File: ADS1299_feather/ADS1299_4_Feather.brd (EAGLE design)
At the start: 90 x 40 mm, 40 parts, among them U1 ADS1299-4PAG

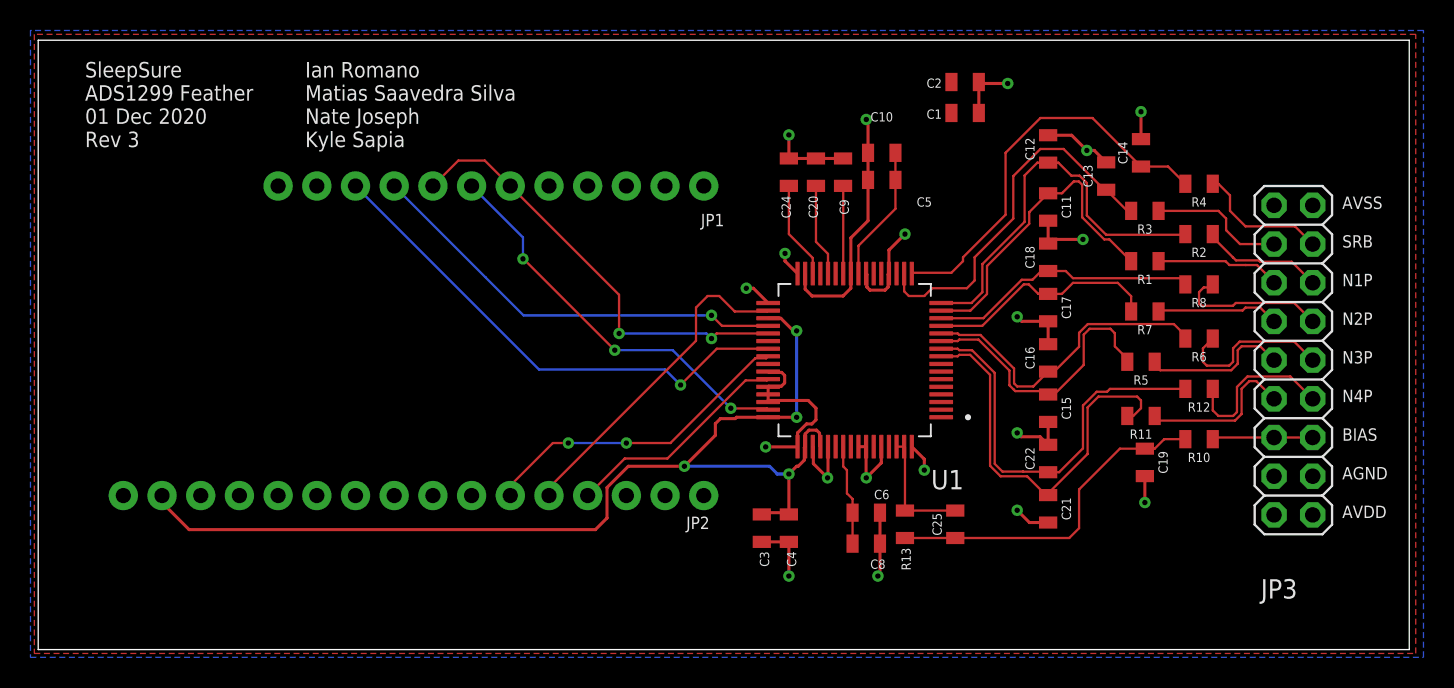
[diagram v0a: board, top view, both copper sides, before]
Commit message: Uploading final standalone and feather files
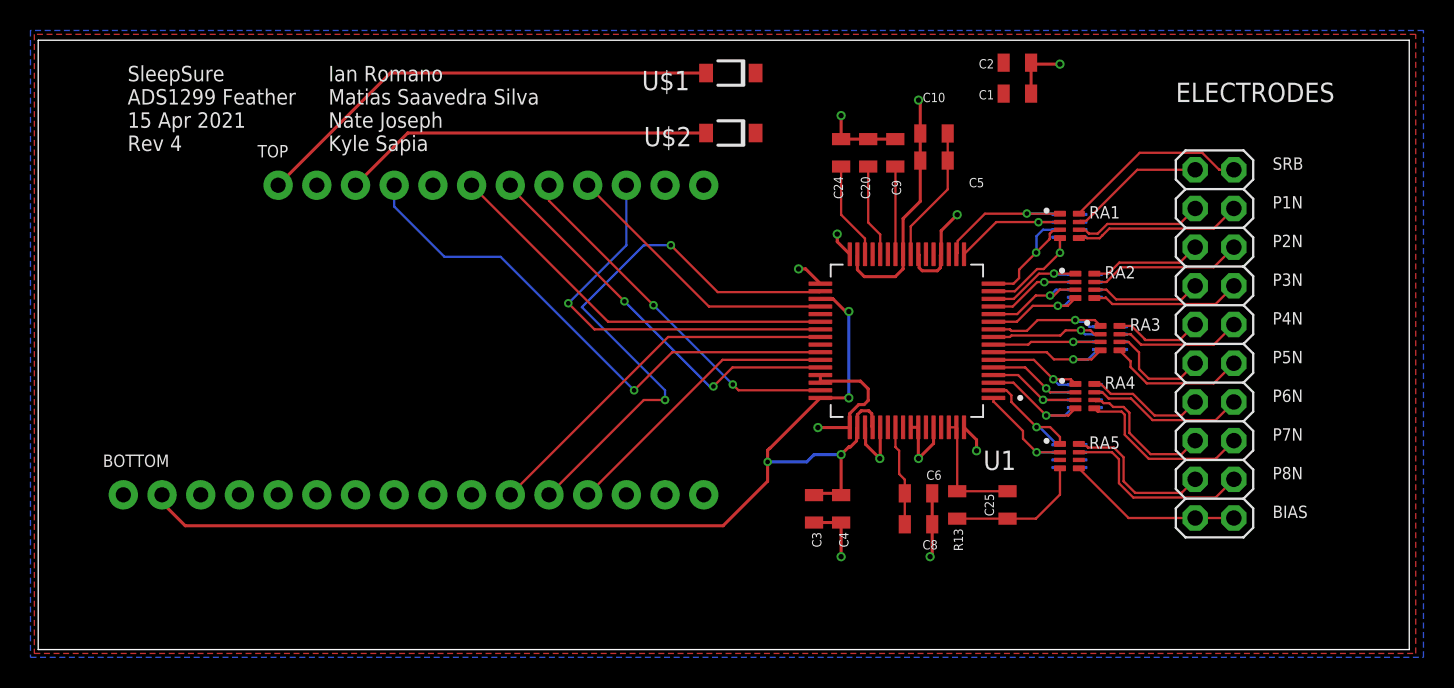
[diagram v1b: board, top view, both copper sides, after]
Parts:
- removed C11, C12, C13, C14, C15, C16, C17, C18, C19, C21, C22: 1nF, SparkFun-Capacitors:0805
- removed JP1: 1x12, Proto FeatherWing:MICROBUILDER_1X12_ROUND_76MIL
- removed JP2: 1x16, Proto FeatherWing:MICROBUILDER_1X16_ROUND_76MIL
- removed JP3: 2x9, adafruit:2X09-BIG
- removed R1, R10, R11, R12, R2, R3, R4, R5, R6, R7, R8: 2.2k, SparkFun-Resistors:0805
- added BOTTOM: (no value), ADS_Feather:MICROBUILDER_1X16_ROUND_76MIL
- added CA1, CA2, CA3, CA4, CA5: 1nF, ADS_Feather:SLEEPSURELIB_CAPCAXE50P210X130X94-8N
- added ELECTRODES: (no value), ADS_Feather:SLEEPSURELIB_2X10-BIG
- added RA1, RA2, RA3, RA4, RA5: 2.2k, ADS_Feather:SLEEPSURELIB_RESCAXS50P200X100X45-8N
- added TOP: (no value), ADS_Feather:MICROBUILDER_1X12_ROUND_76MIL
- added U$1, U$2: MRB120, ADS_Feather:SOD123FL
- moved C10 3.66 mm to (58.8, 33.9)
- moved C5 3.66 mm to (58.8, 32.1)
- moved C25 3.66 mm to (63.6, 9.49)
- moved C3 3.66 mm to (50.9, 9.24)
- moved R13 3.66 mm to (60.3, 9.49)
- moved U1 3.66 mm to (57.0, 20.3)
- moved C9 3.66 mm to (56.3, 32.6)
- moved C2 3.66 mm to (64.3, 38.5)
- moved C4 3.66 mm to (52.7, 9.24)
- moved C8 3.66 mm to (57.8, 8.22)
- moved C6 3.66 mm to (57.8, 10.3)
- moved C1 3.66 mm to (64.3, 36.5)
- moved C20 3.66 mm to (54.5, 32.6)
- moved C24 3.66 mm to (52.7, 32.6)
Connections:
- removed net CLK0: JP1.6, JP1.8, U1.37
- removed net EN: JP1.2
- removed net RESET: JP2.1
- new net 5_N: ELECTRODES.N5, RA3.5
- new net 5_P: ELECTRODES.P5, RA3.6
- new net 6_N: ELECTRODES.N6, RA4.7
- new net 6_P: ELECTRODES.P6, RA4.8
- new net 7_N: ELECTRODES.N7, RA4.5
- new net 7_P: ELECTRODES.P7, RA4.6
- new net 8_N: ELECTRODES.N8, RA5.7
- new net 8_P: ELECTRODES.P8, RA5.8
- new net ADS_START: TOP.27/A10, U1.38
- new net GPIO1: TOP.13/A12, U1.42
- new net GPIO2: TOP.33/A9, U1.44
- new net IN5_N: CA3.1, RA3.4, U1.7
- new net IN5_P: CA3.2, RA3.3, U1.8
- new net IN6_N: CA4.3, RA4.2, U1.5
- new net IN6_P: CA4.4, RA4.1, U1.6
- new net IN7_N: CA4.1, RA4.4, U1.3
- new net IN7_P: CA4.2, RA4.3, U1.4
- new net IN8_N: CA5.3, RA5.2, U1.1
- new net IN8_P: CA5.4, RA5.1, U1.2
- new net USB: TOP.USB, U$2.A
- net 1_N: now also ELECTRODES.N1, RA1.5; no longer JP3.14, R1.1
- net 1_P: now also ELECTRODES.P1, RA1.6; no longer JP3.13, R2.1
- net 2_N: now also ELECTRODES.N2, RA2.7; no longer JP3.12, R7.1
- net 2_P: now also ELECTRODES.P2, RA2.8; no longer JP3.11, R8.1
- net 3V3: now also BOTTOM.3V; no longer JP2.2
- net 3_N: now also ELECTRODES.N3, RA2.5; no longer JP3.10, R5.1
- net 3_P: now also ELECTRODES.P3, RA2.6; no longer JP3.9, R6.1
- net 4_N: now also ELECTRODES.N4, RA3.7; no longer JP3.8, R11.1
- net 4_P: now also ELECTRODES.P4, RA3.8; no longer JP3.7, R12.1
- net 5V: now also U$1.C, U$2.C; no longer JP1.3, JP3.1, JP3.2, U1.1, U1.2, U1.3, U1.4, U1.5, U1.6, U1.7, U1.8
- net ADS_RESET: now also TOP.32/A7; no longer JP1.9
- net BATT: now also TOP.BAT, U$1.A; no longer JP1.1
- net BIAS: now also ELECTRODES.BIAS1, ELECTRODES.BIAS2, RA5.5; no longer JP3.5, JP3.6, R10.1
- net BIAS_DRV: now also RA5.4; no longer C19.1, R10.2
- net CS1: now also TOP.14/A6; no longer JP1.10
- net DRDY: now also TOP.15/A8; no longer JP1.7
- net GND: now also BOTTOM.GND, CA1.5, CA1.6, CA1.7, CA1.8, CA2.5, CA2.6, CA2.7, CA2.8, CA3.5, CA3.6, CA3.7, CA3.8, CA4.5, CA4.6, CA4.7, CA4.8, CA5.5, CA5.6; no longer C11.2, C12.2, C13.2, C14.2, C15.2, C16.2, C17.2, C18.2, C19.2, C21.2, C22.2, JP2.4, JP3.17, JP3.18, JP3.3, JP3.4, U1.42, U1.44
- net IN1_N: now also CA1.1, RA1.4; no longer C11.1, R1.2
- net IN1_P: now also CA1.2, RA1.3; no longer C12.1, R2.2
- net IN2_N: now also CA2.3, RA2.2; no longer C17.1, R7.2
- net IN2_P: now also CA2.4, RA2.1; no longer C18.1, R8.2
- net IN3_N: now also CA2.1, RA2.4; no longer C15.1, R5.2
- net IN3_P: now also CA2.2, RA2.3; no longer C16.1, R6.2
- net IN4_N: now also CA3.3, RA3.2; no longer C21.1, R11.2
- net IN4_P: now also CA3.4, RA3.1; no longer C22.1, R12.2
- net MISO: now also BOTTOM.MISO/19; no longer JP2.13
- net MOSI: now also BOTTOM.MOSI/18; no longer JP2.12
- net SCLK: now also BOTTOM.SCK/5; no longer JP2.11
- net SRB1: now also ELECTRODES.SRB1, RA1.7; no longer JP3.15, R4.1
- net SRB2: now also ELECTRODES.SRB2, RA1.8; no longer JP3.16, R3.1
- net _SRB1: now also CA1.3, RA1.2; no longer C14.1, R4.2
- net _SRB2: now also CA1.4, RA1.1; no longer C13.1, R3.2
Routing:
- net GPIO1: track 0.00 -> 35.4 mm, vias 0 -> 1
- net BATT: track 0.00 -> 31.1 mm
- net CLK0: track 29.2 -> 0.00 mm, vias 2 -> 0
- net ADS_START: track 0.00 -> 26.6 mm
- net GPIO2: track 0.00 -> 26.4 mm, vias 0 -> 2
- net GND: track 89.0 -> 63.9 mm, vias 19 -> 12
- net USB: track 0.00 -> 24.4 mm
- net IN4_N: track 26.7 -> 8.54 mm, vias 0 -> 1
- net _SRB1: track 26.5 -> 8.42 mm, vias 0 -> 1
- net IN4_P: track 26.8 -> 9.20 mm, vias 0 -> 1
- net IN1_P: track 25.9 -> 8.99 mm, vias 0 -> 1
- net MOSI: track 21.8 -> 37.2 mm, vias 0 -> 2
- net _SRB2: track 24.4 -> 10.4 mm, vias 0 -> 1
- net IN1_N: track 20.9 -> 7.47 mm, vias 0 -> 1
- net BIAS_DRV: track 22.6 -> 9.13 mm
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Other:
- board text added: "G:/downloads/struttinYD-blue.bmp"
- board text added: "SleepSure ADS1299 Feather 15 Apr 2021 Rev 4"
- board text removed: "AVSS SRB N1P N2P N3P N4P BIAS AGND AVDD"
- board text removed: "SleepSure ADS1299 Feather 01 Dec 2020 Rev 3"
